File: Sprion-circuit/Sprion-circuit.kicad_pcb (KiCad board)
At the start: 2 copper layers, 107.5 x 72 mm, 117 parts, among them IC1 R3111N211A, IC2 TAR5SB50, IC5 NJU6080F1, IC6 NJU6080F1, IC7 NJU6080F1, IC8 NJU6080F1, J1 Conn_01x03_Female, J2 Conn_01x04_Female, J3 Conn_02x03_Odd_Even, J4 Conn_02x03_Odd_Even, J5 Conn_01x02_Female, J6 Conn_01x04_Female, Q1 IRML6402, Q2 IRML6402, Q3 IRFML8244, Q4 RUE002N02, SW1 SSAJ120100, SW2 SW_Push, SW3 SW_Push, SW4 SW_Push, U1 ICM-20602, U2 INA185, U3 STM32F405RGTx, U4 TLV9061, U5 INA185, U6 TLV9061, U7 TLV9061, U8 TLV9061, U9 LXDC55FAAA-203

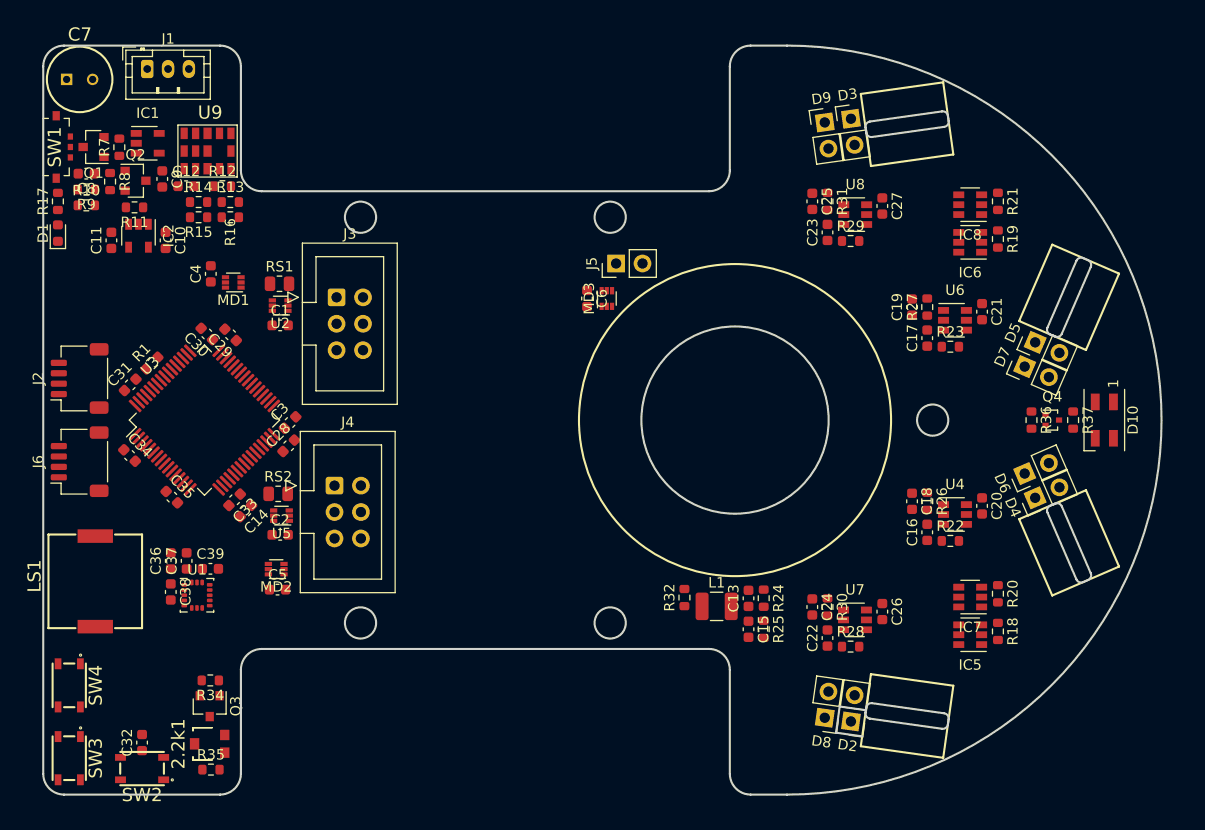
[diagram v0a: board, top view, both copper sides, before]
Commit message: add fix feat: でけたー（コミットしてなくてごめん）
ベタ塗、配線、再配置等
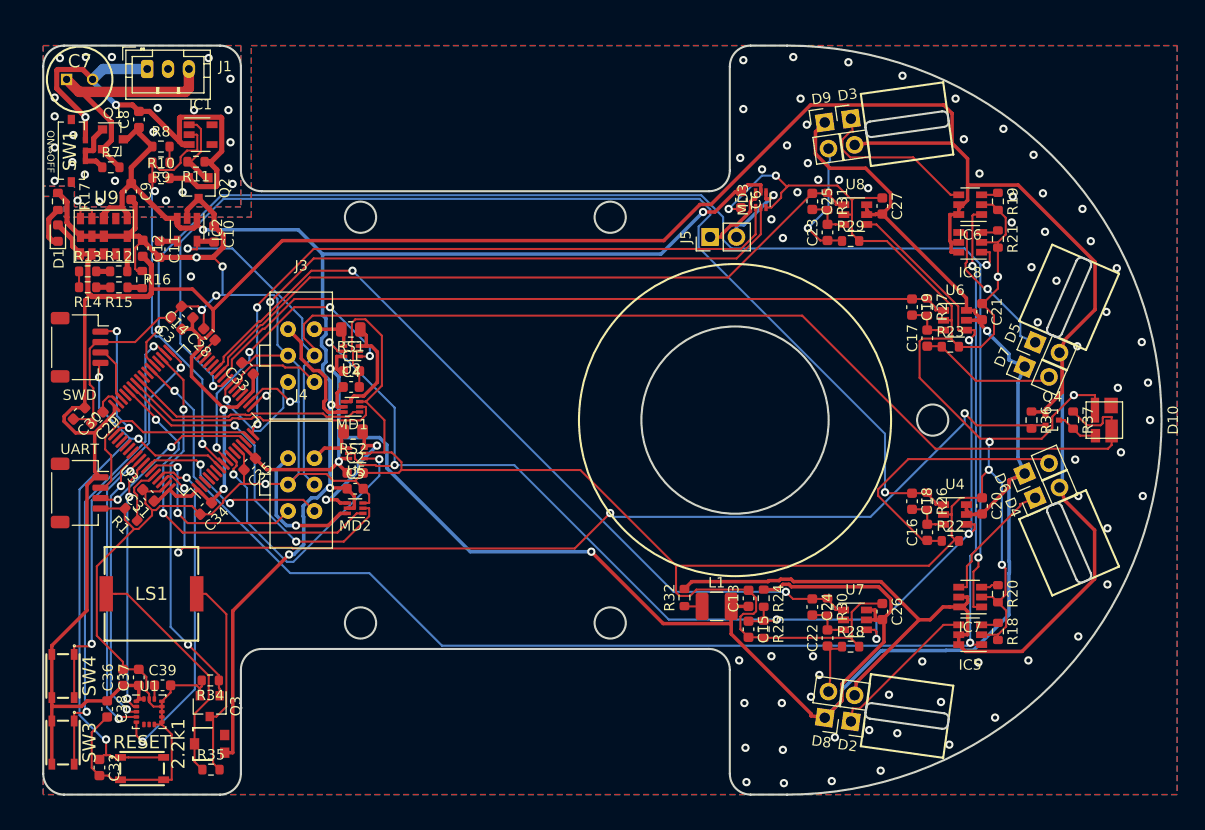
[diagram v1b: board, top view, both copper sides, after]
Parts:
- removed J2: Conn_01x04_Female, Connector_JST:JST_SH_SM04B-SRSS-TB_1x04-1MP_P1.00mm_Horizontal
- added SWD: Conn_01x04_Female, Connector_JST:JST_SH_SM04B-SRSS-TB_1x04-1MP_P1.00mm_Horizontal, F.Cu at (52.0, 72.0)
- D10: footprint LED_SMD:LED_SK6812MINI_PLCC4_3.5x3.5mm_P1.75mm -> Sprion-circuit:SK6812MINI
- J3, J4: footprint Connector_IDC:IDC-Header_2x03_P2.54mm_Vertical -> Sprion-circuit:1717CXR+IE2-4096
- MD1, MD2, MD3, U2, U5: footprint Package_TO_SOT_SMD:SOT-563 -> Sprion-circuit:SOT-563
- Q2: value IRML6402 -> IRFML8244
- moved C14 19.9 mm to (62.3, 68.6), turned to 135 degrees
- moved MD3 17.6 mm to (117.5, 57.8)
- moved C6 17.6 mm to (115.6, 57.8)
- moved C4 17.3 mm to (78.1, 75.8), turned to 0 degrees
- moved MD1 16.5 mm to (78.2, 77.7)
- moved R13 15.2 mm to (52.8, 64.7)
- moved C29 15.1 mm to (53.7, 78.8), turned to 225 degrees
- moved R1 14.7 mm to (56.9, 88.1), turned to 135 degrees
- moved C3 14.5 mm to (61.3, 69.7), turned to 135 degrees
- moved C30 14.5 mm to (51.9, 78.4), turned to 225 degrees
- moved R14 13.4 mm to (52.8, 66.2), turned to 180 degrees
- moved C28 13.1 mm to (64.5, 70.8), turned to 135 degrees
- moved R12 12.9 mm to (55.8, 64.7)
- moved U9 12.9 mm to (56.6, 59.6)
- moved C38 12.8 mm to (54.6, 106.8)
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- renumbered SW2 to RESET, J6 to UART
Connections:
- C7 pad 2: GND -> Net-(C7-Pad2)
- C8 pad 1: Net-(C8-Pad1) -> +BATT
- C8 pad 2: GND -> Net-(C7-Pad2)
- D10 pad 2: GND -> +5V
- D10 pad 4: +5V -> GND
- IC1 pad 3: GND -> Net-(C7-Pad2)
- J1 pad 1: GND -> Net-(C7-Pad2)
- Q1 pad 3: Net-(C8-Pad1) -> +BATT
- Q2 pad 2: Net-(C8-Pad1) -> Net-(C7-Pad2)
- Q2 pad 3: +BATT -> GND
- Q4 pad 3: Net-(D10-Pad3) -> Net-(D10-Pad1)
- R10 pad 2: GND -> Net-(C7-Pad2)
- R11 pad 1: Net-(IC1-Pad1) -> Net-(C7-Pad2)
- R11 pad 2: Net-(C8-Pad1) -> Net-(IC1-Pad1)
- R37 pad 2: Net-(D10-Pad3) -> Net-(D10-Pad1)
- R8 pad 1: Net-(C8-Pad1) -> +BATT
- SW1 pad 1: GND -> Net-(C7-Pad2)
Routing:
- net GND: track 0.00 -> 447.9 mm, vias 0 -> 82
- net +3V3: track 0.00 -> 355.9 mm, vias 0 -> 2
- net +3.3VA: track 0.00 -> 215.2 mm, vias 0 -> 4
- net +BATT: track 0.00 -> 145.5 mm, vias 0 -> 5
- net /Controller/IRLED_SIDE: track 0.00 -> 137.1 mm, vias 0 -> 3
- net /Controller/IRLED_FRONT: track 0.00 -> 133.4 mm, vias 0 -> 3
- net VREF: track 0.00 -> 131.8 mm, vias 0 -> 6
- net +5V: track 0.00 -> 129.0 mm, vias 0 -> 1
- net /Controller/SENSOR_WALL_FR: track 0.00 -> 111.2 mm, vias 0 -> 2
- net /Controller/FULLCOLOR_LED: track 0.00 -> 99.9 mm, vias 0 -> 4
- net /Controller/SENSOR_WALL_SR: track 0.00 -> 78.2 mm, vias 0 -> 2
- net /Controller/SENSOR_WALL_FL: track 0.00 -> 73.5 mm
- net /Controller/SENSOR_WALL_SL: track 0.00 -> 68.2 mm
- net /Controller/MD_SUC_IN1: track 0.00 -> 65.9 mm, vias 0 -> 2
- net /Controller/MD_SUC_IN2: track 0.00 -> 63.3 mm, vias 0 -> 2
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- added copper zone on B.Cu, net GND
- added copper zone on F.Cu, net GND
- added copper zone on B.Cu, net Net-(C7-Pad2)
- added copper zone on F.Cu, net Net-(C7-Pad2)
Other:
- outline, holes or cut-outs redrawn
- net class Default: clearance 0.2 -> 0.1524; trace_width 0.25 -> 0.2
- net class Power added: clearance 0.1524, trace_width 0.34, via_dia 0.8, via_drill 0.4
- rule trace_clearance: 0.2 -> 0.1524
- board text added: "ON⇔OFF"
